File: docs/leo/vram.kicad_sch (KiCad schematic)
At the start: 2 parts, among them IC25 UPD43256AC-10L, IC26 UPD43256AC-10L

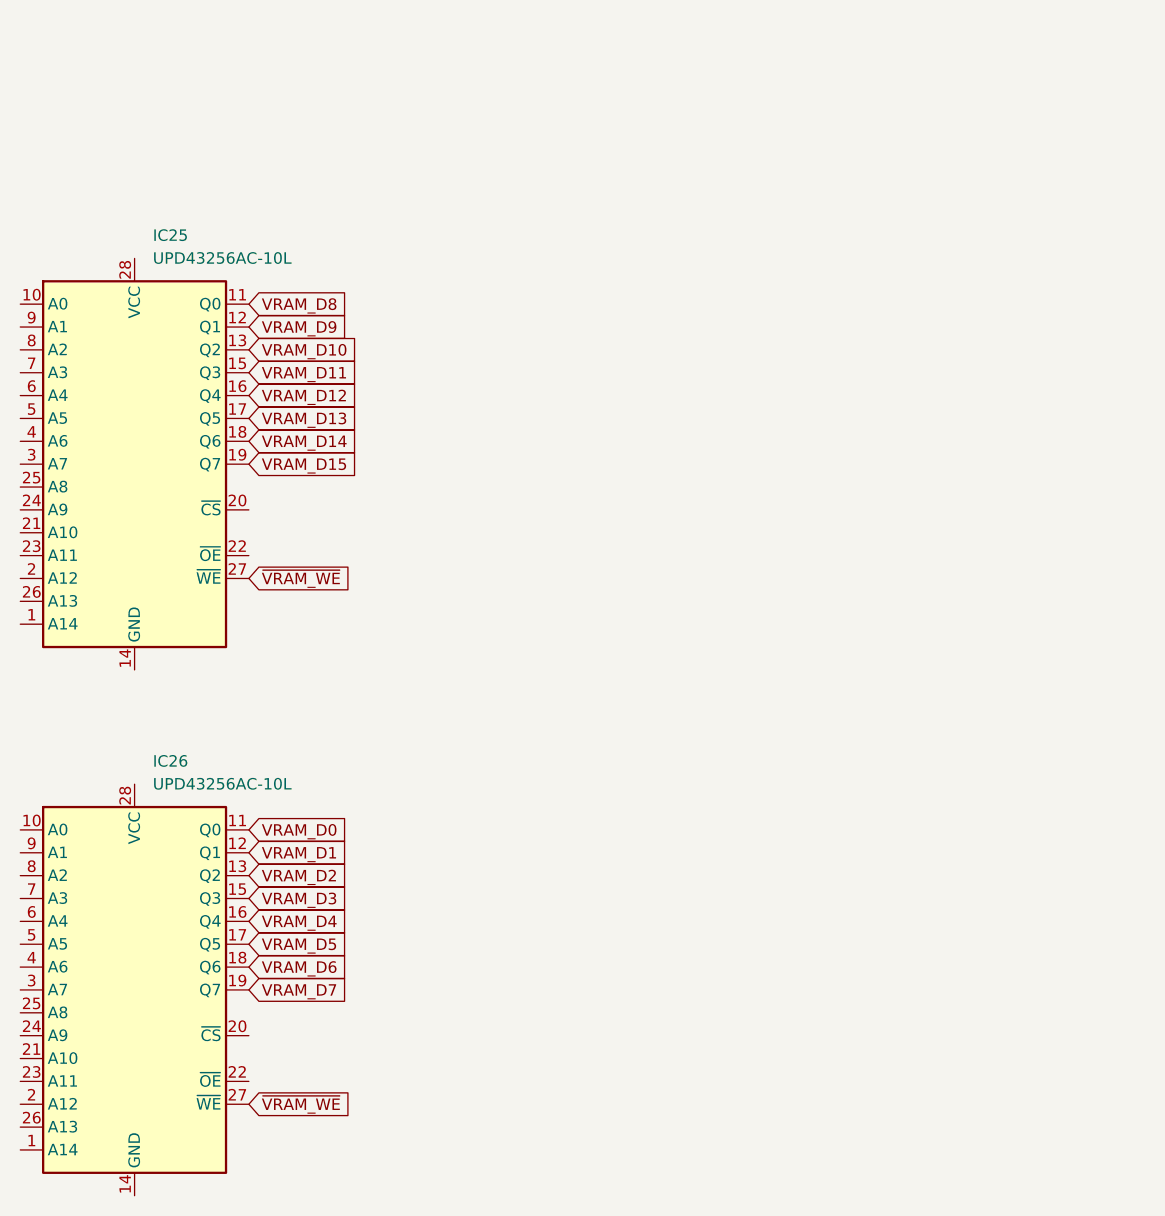
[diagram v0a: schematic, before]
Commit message: Add more b board logic
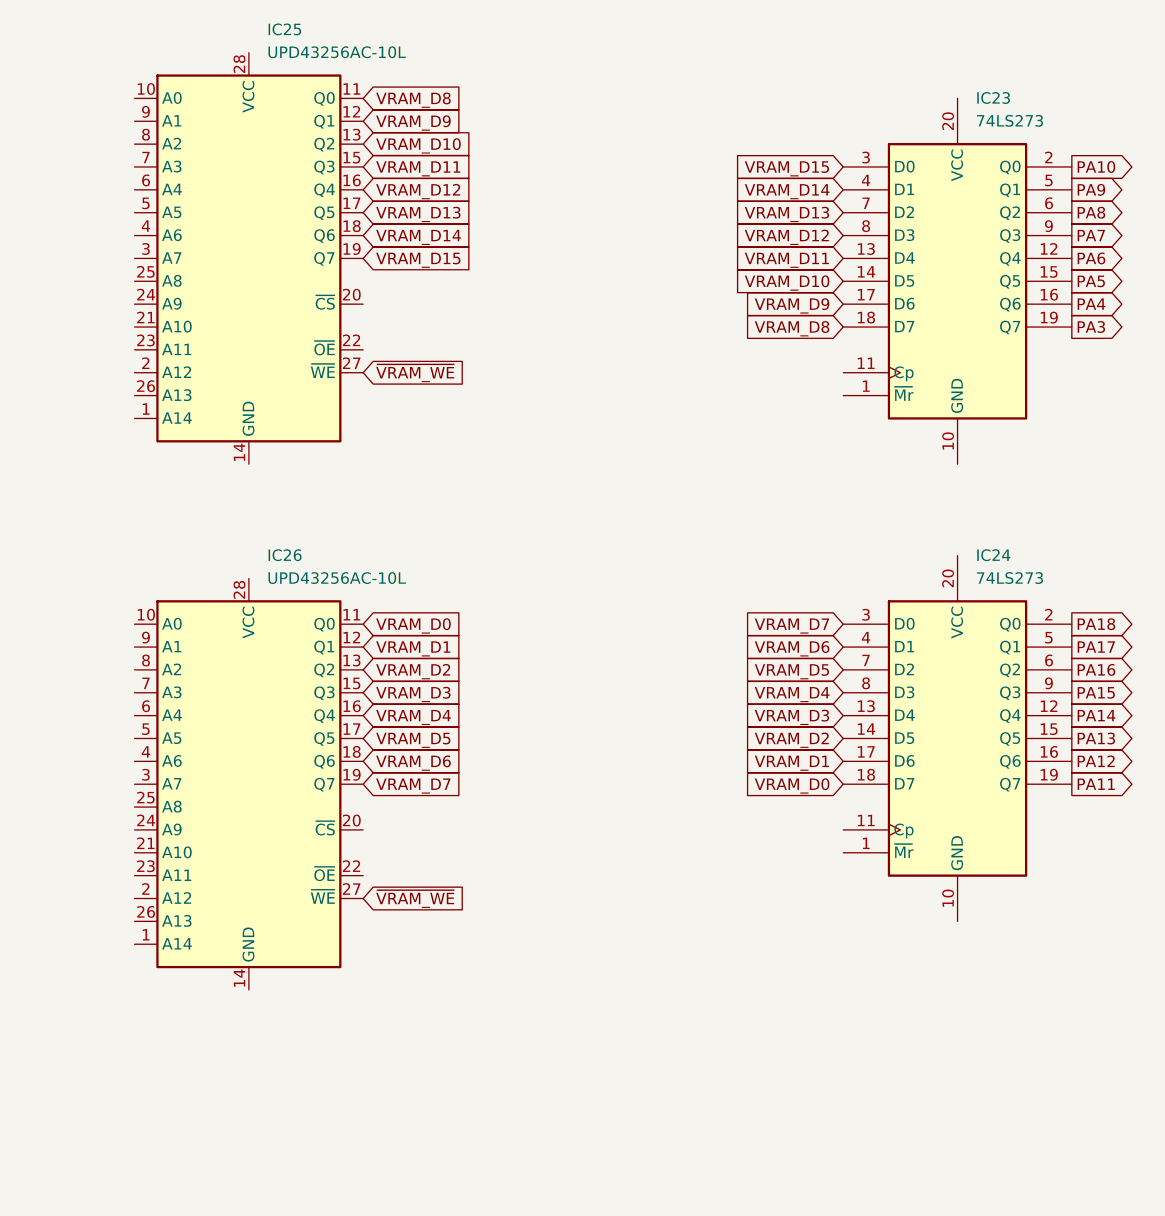
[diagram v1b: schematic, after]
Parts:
- added IC23, IC24: 74LS273, symbol 74xx:74LS273
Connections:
- net VRAM_D0: now also IC24.18 (D7)
- net VRAM_D1: now also IC24.17 (D6)
- net VRAM_D10: now also IC23.14 (D5)
- net VRAM_D11: now also IC23.13 (D4)
- net VRAM_D12: now also IC23.8 (D3)
- net VRAM_D13: now also IC23.7 (D2)
- net VRAM_D14: now also IC23.4 (D1)
- net VRAM_D15: now also IC23.3 (D0)
- net VRAM_D2: now also IC24.14 (D5)
- net VRAM_D3: now also IC24.13 (D4)
- net VRAM_D4: now also IC24.8 (D3)
- net VRAM_D5: now also IC24.7 (D2)
- net VRAM_D6: now also IC24.4 (D1)
- net VRAM_D7: now also IC24.3 (D0)
- net VRAM_D8: now also IC23.18 (D7)
- net VRAM_D9: now also IC23.17 (D6)
- new net PA10: IC23.2 (Q0)
- new net PA11: IC24.19 (Q7)
- new net PA12: IC24.16 (Q6)
- new net PA13: IC24.15 (Q5)
- new net PA14: IC24.12 (Q4)
- new net PA15: IC24.9 (Q3)
- new net PA16: IC24.6 (Q2)
- new net PA17: IC24.5 (Q1)
- new net PA18: IC24.2 (Q0)
- new net PA3: IC23.19 (Q7)
- new net PA4: IC23.16 (Q6)
- new net PA5: IC23.15 (Q5)
- new net PA6: IC23.12 (Q4)
- new net PA7: IC23.9 (Q3)
- new net PA8: IC23.6 (Q2)
- new net PA9: IC23.5 (Q1)
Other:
- moved on the sheet: IC25, IC26
